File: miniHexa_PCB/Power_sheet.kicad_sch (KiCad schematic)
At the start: 34 parts, among them J2 12v DC, U3 RT8289GSP, U4 BQ25886RGE, U6 AMS1117-3.3

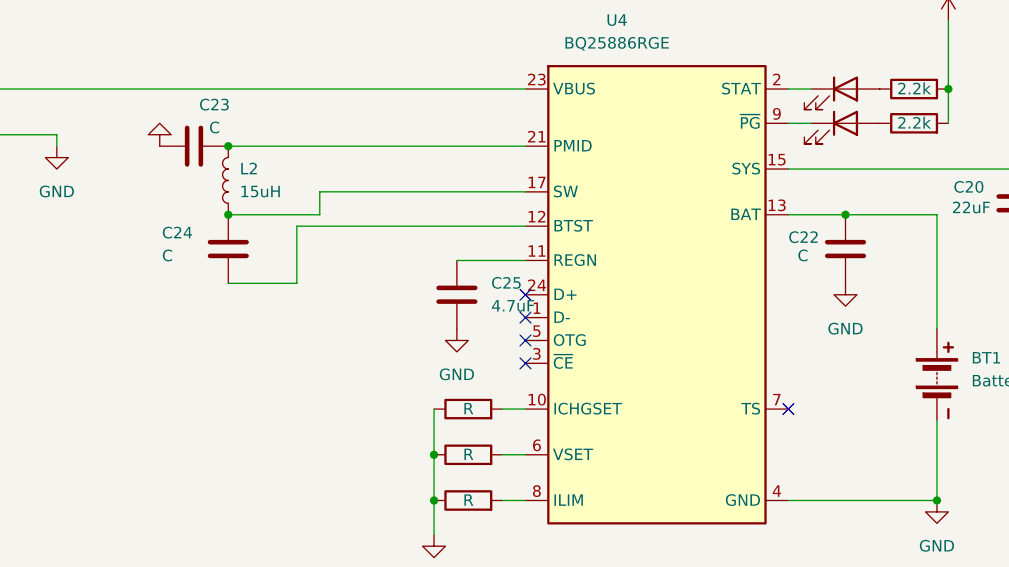
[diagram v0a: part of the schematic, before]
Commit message: layout phase pcb
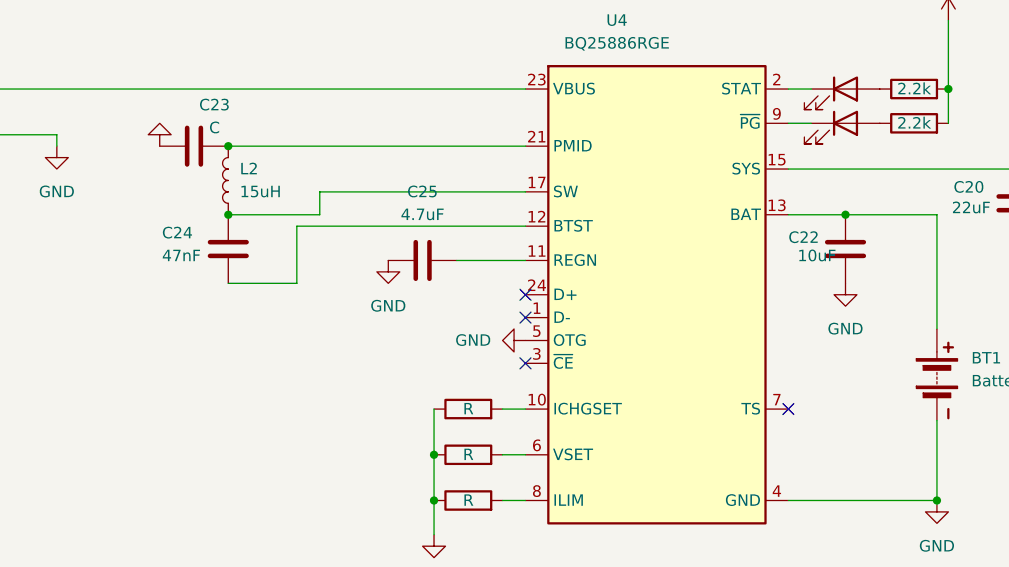
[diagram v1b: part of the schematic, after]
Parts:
- C19: footprint Capacitor_SMD:C_0402_1005Metric -> Capacitor_SMD:CP_Elec_6.3x7.7
- C22: value C -> 10uF
- C24: value C -> 47nF
- R22, R23, R24, R25, R26, R27, R28, R30, R31: footprint Resistor_SMD:R_0805_2012Metric -> Resistor_SMD:R_0402_1005Metric
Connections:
- net GND: now also C25.1, U4.5 (OTG); no longer C25.2
- net at U4.11 (REGN): now also C25.2; no longer C25.1
- no-connect marks 7 -> 6
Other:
- moved on the sheet: C25
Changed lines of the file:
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@@
 		(at 203.2 59.69)
 	)
-	(no_connect
-		(at 203.2 64.77)
-	)
 	(wire
 		(pts
@@
 			)
 		)
-		(property "Footprint" "Resistor_SMD:R_0805_2012Metric"
+		(property "Footprint" "Resistor_SMD:R_0402_1005Metric"
 			(at 65.532 38.1 90)
 			(hide yes)
@@
 			)
 		)
-		(property "Footprint" "Resistor_SMD:R_0805_2012Metric"
+		(property "Footprint" "Resistor_SMD:R_0402_1005Metric"
 			(at 246.38 38.608 90)
 			(hide yes)
@@
 			)
 		)
-		(property "Footprint" "Resistor_SMD:R_0805_2012Metric"
+		(property "Footprint" "Resistor_SMD:R_0402_1005Metric"
 			(at 196.85 84.328 90)
 			(hide yes)
@@
 	(symbol
 		(lib_id "power:GND")
+		(at 203.2 64.77 270)
+		(unit 1)
+		(body_style 1)
+		(exclude_from_sim no)
+		(in_bom yes)
+		(on_board yes)
+		(in_pos_files yes)
+		(dnp no)
+		(fields_autoplaced yes)
+		(property "Reference" "#PWR032"
+			(at 196.85 64.77 0)
+			(hide yes)
+			(show_name no)
+			(do_not_autoplace no)
+			(effects
+				(font
+					(size 1.27 1.27)
+				)
+			)
+		)
+		(property "Value" "GND"
+			(at 199.39 64.7699 90)
+			(show_name no)
+			(do_not_autoplace no)
+			(effects
+				(font
+					(size 1.27 1.27)
+				)
+				(justify right)
+			)
+		)
+		(property "Footprint" ""
+			(at 203.2 64.77 0)
+			(hide yes)
+			(show_name no)
+			(do_not_autoplace no)
+			(effects
+				(font
+					(size 1.27 1.27)
+				)
+			)
+		)
+		(property "Datasheet" ""
+			(at 203.2 64.77 0)
+			(hide yes)
+			(show_name no)
+			(do_not_autoplace no)
+			(effects
+				(font
+					(size 1.27 1.27)
+				)
+			)
+		)
+		(property "Description" "Power symbol creates a global label with name \"GND\" , ground"
+			(at 203.2 64.77 0)
+			(hide yes)
+			(show_name no)
+			(do_not_autoplace no)
+			(effects
+				(font
+					(size 1.27 1.27)
+				)
+			)
+		)
+		(pin "1"
+		)
+		(instances
+			(project "miniHexa"
+				(path "/3449ee66-2977-4802-a474-0821cdf4e79b/33698118-31e2-44d0-a5be-b46ca646d44a"
+					(reference "#PWR032")
+					(unit 1)
+				)
+			)
+		)
+	)
+	(symbol
+		(lib_id "power:GND")
 		(at 238.76 58.42 0)
 		(unit 1)
@@
 			)
 		)
-		(property "Value" "C"
+		(property "Value" "10uF"
 			(at 233.426 55.372 0)
 			(show_name no)
@@
 	(symbol
 		(lib_id "Device:C")
-		(at 195.58 59.69 0)
+		(at 191.77 55.88 90)
 		(unit 1)
 		(body_style 1)
@@
 		(fields_autoplaced yes)
 		(property "Reference" "C25"
-			(at 199.39 58.4199 0)
+			(at 191.77 48.26 90)
 			(show_name no)
 			(do_not_autoplace no)
@@
 					(size 1.27 1.27)
 				)
-				(justify left)
 			)
 		)
 		(property "Value" "4.7uF"
-			(at 199.39 60.9599 0)
+			(at 191.77 50.8 90)
 			(show_name no)
 			(do_not_autoplace no)
@@
 					(size 1.27 1.27)
 				)
-				(justify left)
 			)
 		)
 		(property "Footprint" "Capacitor_SMD:C_0402_1005Metric"
-			(at 196.5452 63.5 0)
+			(at 195.58 54.9148 0)
 			(hide yes)
 			(show_name no)
@@
 		)
 		(property "Datasheet" ""
-			(at 195.58 59.69 0)
+			(at 191.77 55.88 0)
 			(hide yes)
 			(show_name no)
@@
 		)
 		(property "Description" "Unpolarized capacitor"
-			(at 195.58 59.69 0)
+			(at 191.77 55.88 0)
 			(hide yes)
 			(show_name no)
@@
 			)
 		)
-		(property "Footprint" "Resistor_SMD:R_0805_2012Metric"
+		(property "Footprint" "Resistor_SMD:R_0402_1005Metric"
 			(at 246.38 42.418 90)
 			(hide yes)
@@
 			)
 		)
-		(property "Footprint" "Resistor_SMD:R_0805_2012Metric"
+		(property "Footprint" "Resistor_SMD:R_0402_1005Metric"
 			(at 71.882 162.56 90)
 			(hide yes)
@@
 	(symbol
 		(lib_id "power:GND")
-		(at 195.58 63.5 0)
+		(at 187.96 55.88 0)
 		(unit 1)
 		(body_style 1)
@@
 		(fields_autoplaced yes)
 		(property "Reference" "#PWR031"
-			(at 195.58 69.85 0)
+			(at 187.96 62.23 0)
 			(hide yes)
 			(show_name no)
@@
 		)
 		(property "Value" "GND"
-			(at 195.58 68.58 0)
+			(at 187.96 60.96 0)
 			(show_name no)
 			(do_not_autoplace no)
@@
 		)
 		(property "Footprint" ""
-			(at 195.58 63.5 0)
+			(at 187.96 55.88 0)
 			(hide yes)
 			(show_name no)
@@
 		)
 		(property "Datasheet" ""
-			(at 195.58 63.5 0)
+			(at 187.96 55.88 0)
 			(hide yes)
 			(show_name no)
@@
 		)
 		(property "Description" "Power symbol creates a global label with name \"GND\" , ground"
-			(at 195.58 63.5 0)
+			(at 187.96 55.88 0)
 			(hide yes)
 			(show_name no)
@@
 			)
 		)
-		(property "Footprint" "Resistor_SMD:R_0805_2012Metric"
+		(property "Footprint" "Resistor_SMD:R_0402_1005Metric"
 			(at 71.882 147.32 90)
 			(hide yes)
@@
 			)
 		)
-		(property "Footprint" "Resistor_SMD:R_0805_2012Metric"
+		(property "Footprint" "Resistor_SMD:R_0402_1005Metric"
 			(at 125.73 106.172 90)
 			(hide yes)
@@
 			)
 		)
-		(property "Footprint" "Resistor_SMD:R_0805_2012Metric"
+		(property "Footprint" "Resistor_SMD:R_0402_1005Metric"
 			(at 196.85 79.248 90)
 			(hide yes)
@@
 			)
 		)
-		(property "Footprint" "Capacitor_SMD:C_0402_1005Metric"
+		(property "Footprint" "Capacitor_SMD:CP_Elec_6.3x7.7"
 			(at 39.0652 158.75 0)
 			(hide yes)
@@
 			)
 		)
-		(property "Footprint" "Resistor_SMD:R_0805_2012Metric"
+		(property "Footprint" "Resistor_SMD:R_0402_1005Metric"
 			(at 196.85 74.168 90)
 			(hide yes)
@@
 			)
 		)
-		(property "Value" "C"
+		(property "Value" "47nF"
 			(at 162.814 55.372 0)
 			(show_name no)
